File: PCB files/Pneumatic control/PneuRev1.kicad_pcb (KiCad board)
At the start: 2 copper layers, 230.9 x 92.9 mm, 52 parts, among them J1 SIG_IN, J2 BATT_IN, J3 PNEU, U1 uA7824, U2 OP279, U3 OP279, U4 OP279, U5 OP279, U6 OP279, U7 OP279, U8 OP07

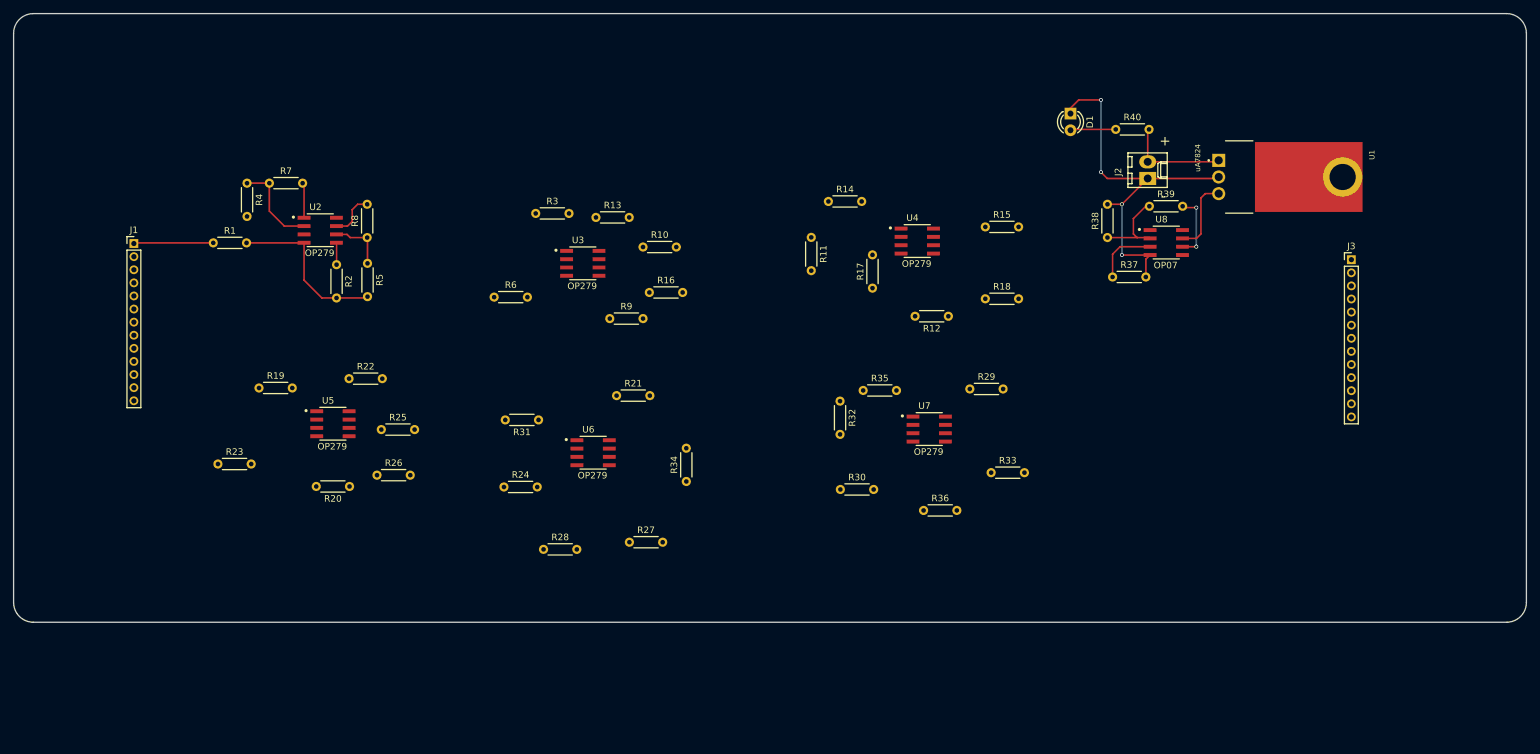
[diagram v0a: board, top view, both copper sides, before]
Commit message: 1/31/2019
-Continued routing board
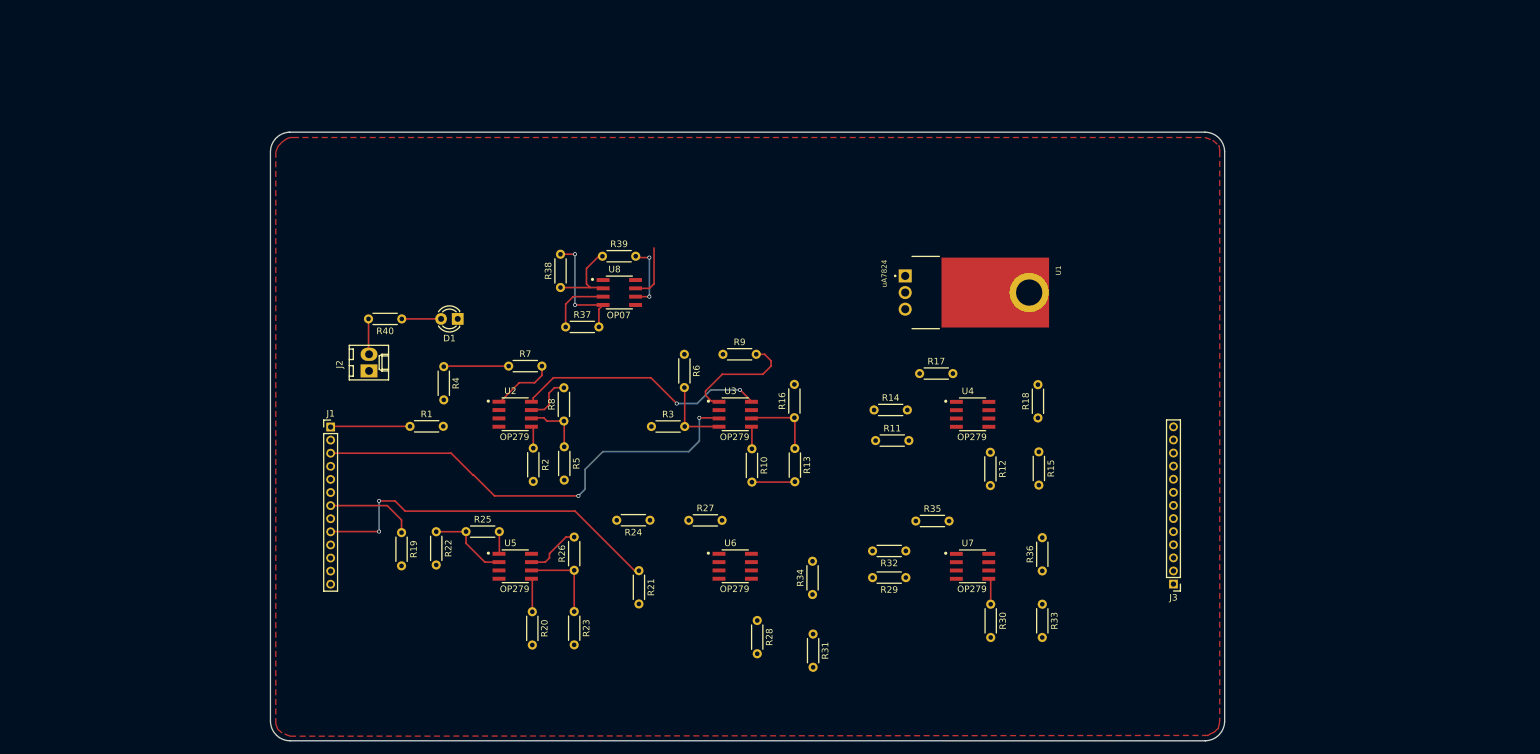
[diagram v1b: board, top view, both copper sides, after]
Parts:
- moved J2 122.4 mm to (89.3, 82.6)
- moved R40 112.8 mm to (94.3, 74.6), turned to 180 degrees
- moved D1 98.7 mm to (102.9, 74.6), turned to 180 degrees
- moved R38 83.8 mm to (118.5, 69.8)
- moved R39 83.8 mm to (124.9, 65.1)
- moved U8 83.8 mm to (127.5, 70.6)
- moved R37 83.8 mm to (119.3, 75.9)
- moved R23 58.9 mm to (120.6, 119.3), turned to 270 degrees
- moved J3 56.5 mm to (212.1, 115.1), turned to 180 degrees
- moved R31 53.1 mm to (157.1, 122.7), turned to 270 degrees
- moved U1 51.0 mm to (171.2, 68.1)
- moved R13 46.5 mm to (154.3, 94.4), turned to 270 degrees
- moved R7 46.0 mm to (110.6, 81.8)
- moved J1 41.1 mm to (83.4, 91.1)
- moved R1 41.1 mm to (95.6, 91.0)
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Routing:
- net /IN3: track 0.00 -> 70.8 mm, vias 0 -> 2
- net /IN9: track 0.00 -> 56.2 mm, vias 0 -> 2
- net GND: track 84.6 -> 36.1 mm, vias 4 -> 2
- net Net-(U1-Pad3): track 11.6 -> 46.9 mm, vias 0 -> 2
- net /PNU3: track 0.00 -> 18.2 mm
- net /IN7: track 0.00 -> 13.7 mm
- net Net-(R23-Pad1): track 0.00 -> 12.8 mm
- net Net-(R22-Pad1): track 0.00 -> 12.6 mm
- net Net-(R13-Pad1): track 0.00 -> 11.3 mm
- net Net-(J2-Pad2): track 16.1 -> 5.43 mm
- net /PNU8: track 0.00 -> 8.50 mm
- net /IN8: track 0.00 -> 5.09 mm
- net /IN12: track 0.00 -> 4.00 mm
- net Net-(R4-Pad1): track 14.0 -> 10.0 mm
- net /PNU1: track 5.37 -> 9.34 mm
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- added copper zone on F.Cu, net GND
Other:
- board size 230.9 x 92.9 mm -> 145.7 x 92.9 mm
- board text removed: "+"
- board text removed: "-"
